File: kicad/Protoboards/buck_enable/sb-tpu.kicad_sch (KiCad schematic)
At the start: 0 parts

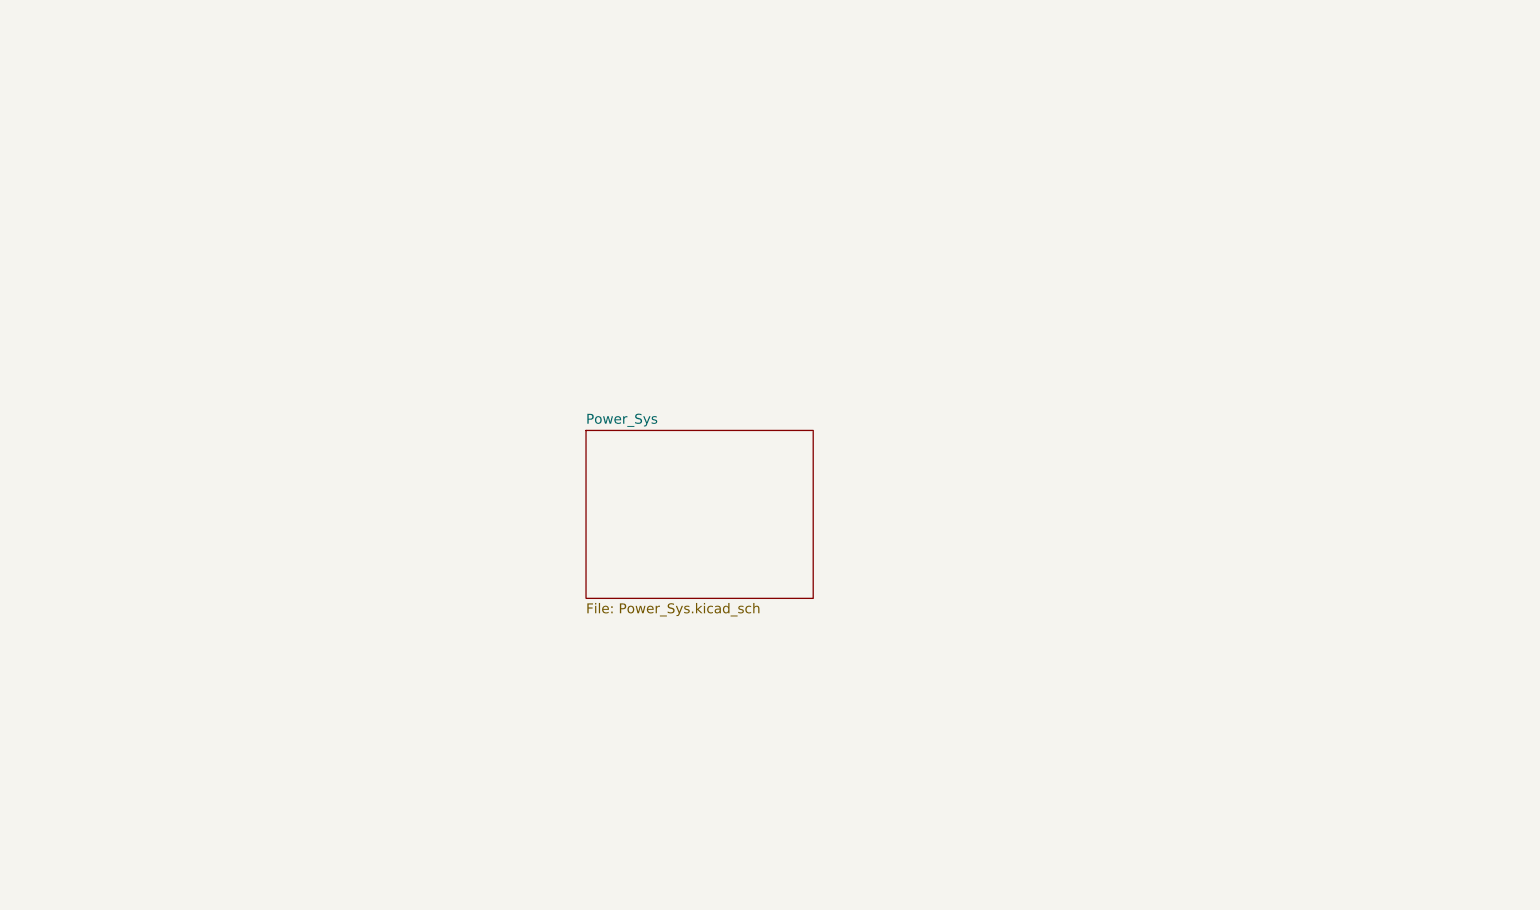
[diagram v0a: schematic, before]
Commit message: [PROTOTYPES] Protoboard layout completed
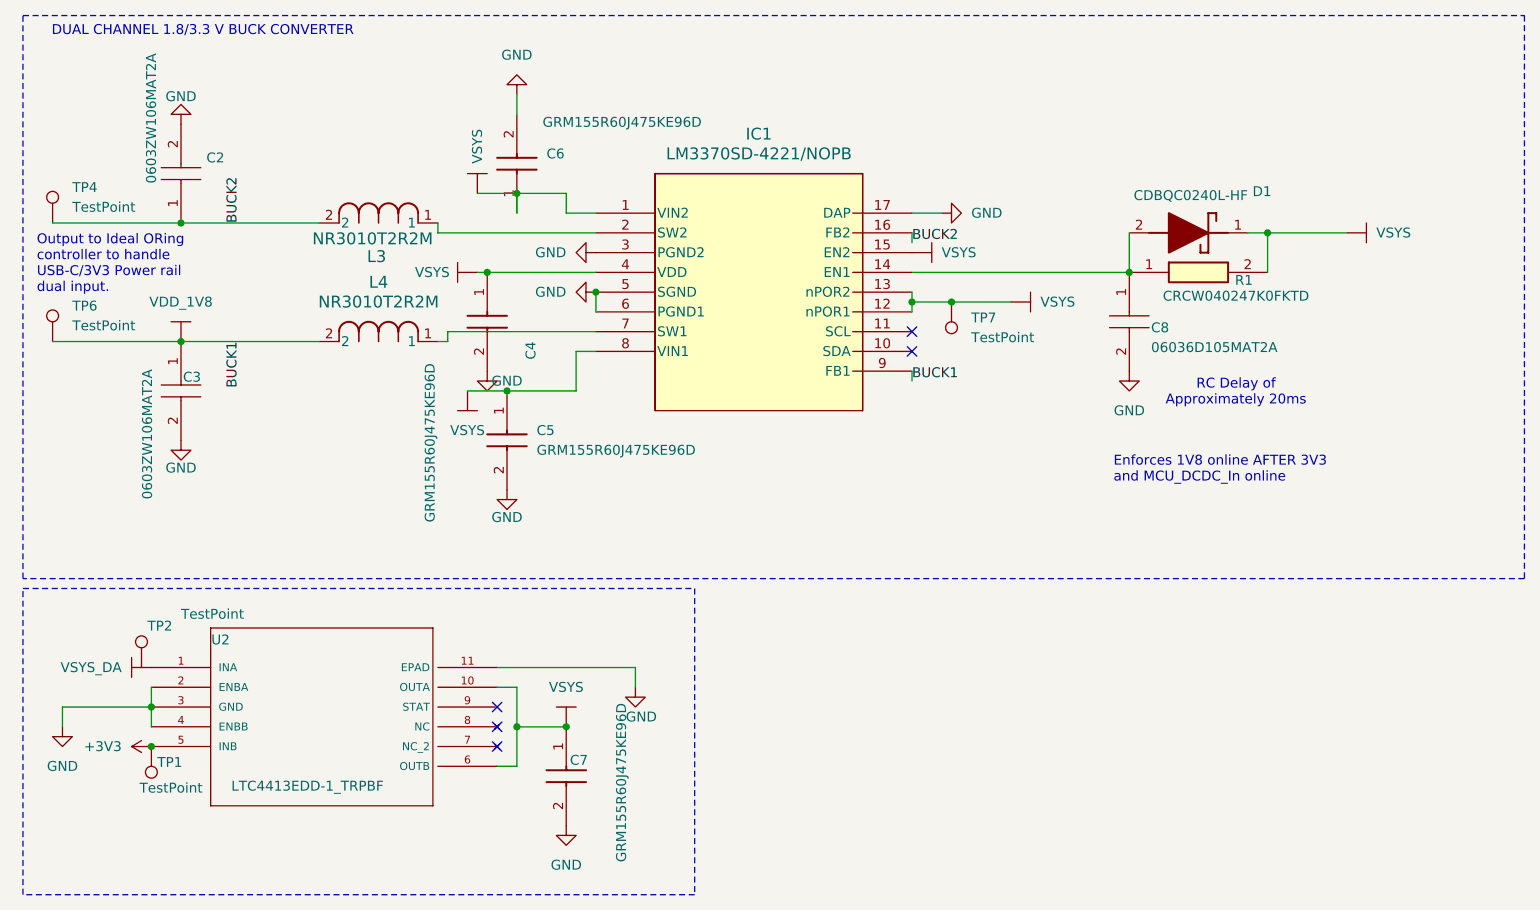
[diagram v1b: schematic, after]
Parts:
- added C2, C3: 0603ZW106MAT2A, footprints:CAPC1608X90N, symbol sb-tpu:0603ZW106MAT2A
- added C4, C5, C6, C7: GRM155R60J475KE96D, footprints:CAPC1005X70N, symbol sb-tpu:GRM155R60J475KE96D
- added C8: 06036D105MAT2A, footprints:CAPC1608X90N, symbol sb-tpu:06036D105MAT2A
- added D1: CDBQC0240L-HF, footprints:CDBQC0240LHF, symbol sb-tpu:CDBQC0240L-HF
- added IC1: LM3370SD-4221/NOPB, footprints:SDA16B, symbol sb-tpu:LM3370SD-4221_NOPB
- added L3, L4: NR3010T2R2M, footprints:IND_TAIYO_NR3010_TAY, symbol sb-tpu:NR3010T2R2M
- added R1: CRCW040247K0FKTD, footprints:CRCW0402200KFKED, symbol sb-tpu:CRCW040247K0FKTD
- added TP1, TP2, TP4, TP6, TP7: TestPoint, TestPoint:TestPoint_Pad_D2.0mm, symbol Connector:TestPoint
- added U2: LTC4413EDD-1_TRPBF, footprints:DFN-10_DD, symbol sb-tpu:LTC4413EDD-1_TRPBF
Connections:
- new net: C8.1, D1.2 (A), IC1.14 (EN1), R1.1
- new net: IC1.2 (SW2), L3.1
- new net: IC1.7 (SW1), L4.1
- new net +3V3: TP1.1, U2.5 (INB)
- new net BUCK2: C2.1, IC1.16 (FB2), L3.2, TP4.1
- new net GND: C2.2, C3.2, C4.2, C5.2, C6.2, C7.2, C8.2, IC1.17 (DAP), IC1.3 (PGND2), IC1.5 (SGND), IC1.6 (PGND1), U2.11 (EPAD), U2.2 (ENBA), U2.3 (GND), U2.4 (ENBB)
- new net VDD_1V8: C3.1, IC1.9 (FB1), L4.2, TP6.1
- new net VSYS: C4.1, C5.1, C6.1, C7.1, D1.1 (K), IC1.1 (VIN2), IC1.12 (nPOR1), IC1.13 (nPOR2), IC1.15 (EN2), IC1.4 (VDD), IC1.8 (VIN1), R1.2, TP7.1, U2.10 (OUTA), U2.6 (OUTB)
- new net VSYS_DA: U2.1 (INA)
- no-connect marks 0 -> 5
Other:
- removed sheet Power_Sys
- note added: "DUAL CHANNEL 1.8/3.3 V BUCK CONVERTER"
- note added: "Enforces 1V8 online AFTER 3V3 and MCU_DCDC_In online"
- note added: "Output to Ideal ORing controller to handle USB-C/3V3 Power rail dual input."
- note added: "RC Delay of Approximately 20ms"
